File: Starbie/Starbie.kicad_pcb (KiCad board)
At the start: 2 copper layers, 114.5 x 104 mm, 7 parts, among them J1 Conn_01x04_Pin, J2 Conn_01x08_Pin, SW1 SW_Push, SW2 SW_Push, U1 XIAO-ESP32-C3-SMD, U2 DHT11

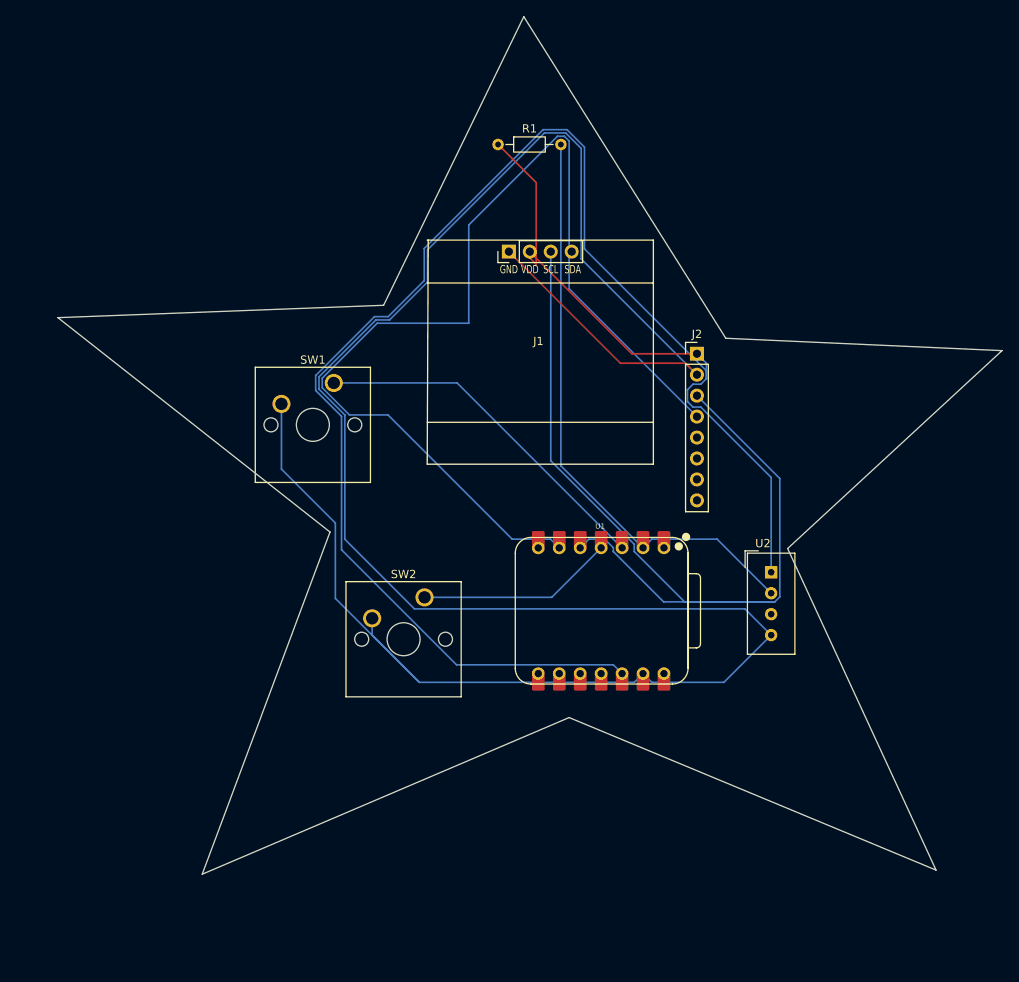
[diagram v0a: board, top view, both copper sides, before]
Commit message: re routed and added art
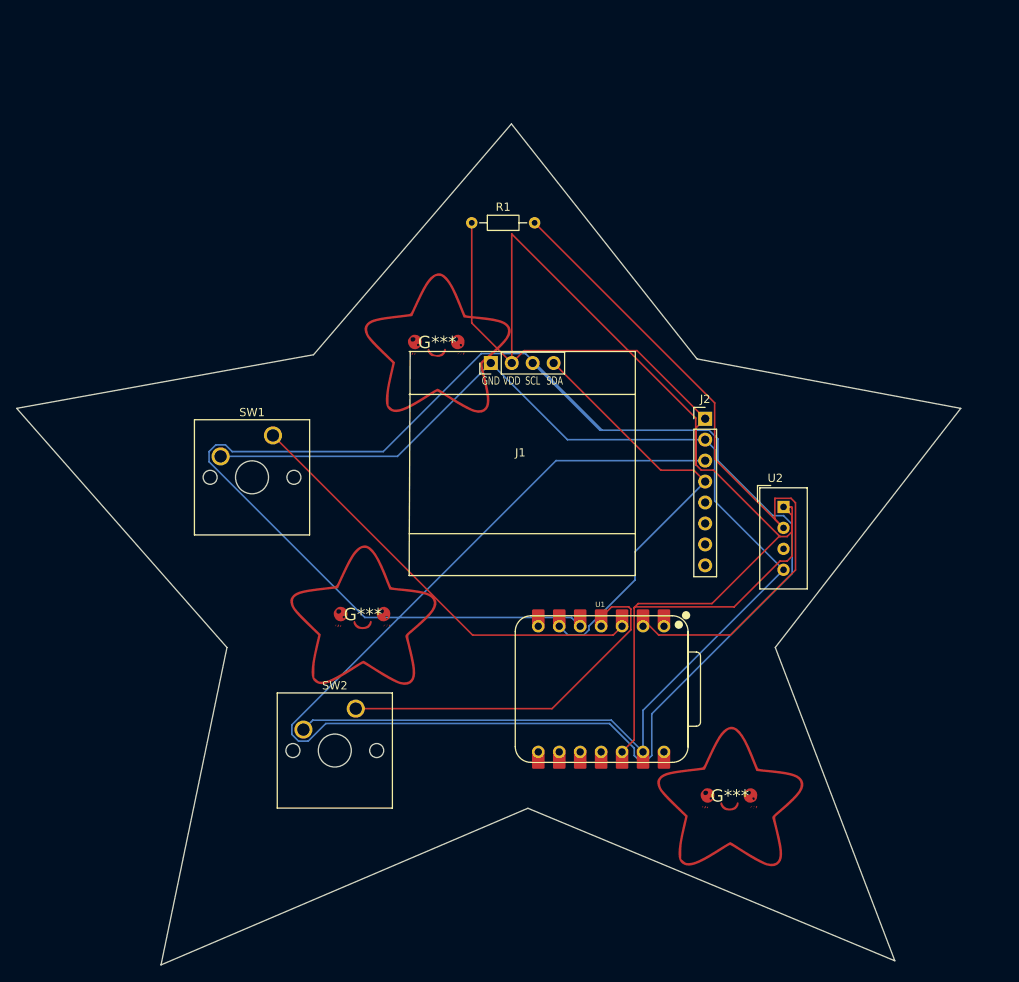
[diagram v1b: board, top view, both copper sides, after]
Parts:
- added G***: LOGO, LOGO, F.Cu at (101.0, 119.5)
- added G***: LOGO, LOGO, F.Cu at (110.0, 86.5)
- added G***: LOGO, LOGO, F.Cu at (145.5, 141.5)
- moved SW2 15.9 mm to (100.1, 130.9)
- moved J1 13.7 mm to (120.3, 89.0)
- moved R1 10.0 mm to (114.2, 72.0)
- moved SW1 9.74 mm to (90.1, 97.8)
- moved U1 9.50 mm to (129.9, 128.5)
- moved U2 8.06 mm to (152.0, 106.5)
- moved J2 7.94 mm to (142.5, 95.8)
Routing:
- net /SCL: track 117.0 -> 300.1 mm
- net GND: track 283.6 -> 159.4 mm
- net /SDA: track 127.1 -> 52.5 mm
- net +3.3V: track 222.1 -> 192.5 mm
- net /GPIO3: track 23.9 -> 45.2 mm
- net /DHT11 DATA: track 71.7 -> 87.0 mm
- net /GPI02: track 43.2 -> 52.8 mm
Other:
- board size 114.5 x 104 mm -> 114.5 x 102 mm
